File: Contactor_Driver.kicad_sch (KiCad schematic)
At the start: 26 parts, among them J1 Conn_01x04, Q3 BUK9M23-80E, Q4 FDC2512, Q5 NTR4003NT1G, Q6 NMOS, U2 SI8261ABC-IS

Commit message: Added part numbers and datasheet to isolator part
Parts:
- Q5: P/N (none) -> NTR4003NT1G
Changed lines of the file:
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@@
       (effects (font (size 1.27 1.27)) hide)
     )
-    (property "Datasheet" "~" (at 50.8 77.47 0)
+    (property "Datasheet" "https://www.mouser.com/datasheet/2/308/1/NTR4003N_D-2319203.pdf" (at 50.8 77.47 0)
       (effects (font (size 1.27 1.27)) hide)
     )
+    (property "P/N" "NTR4003NT1G" (at 50.8 77.47 0)
+      (effects (font (size 1.27 1.27)) hide)
+    )

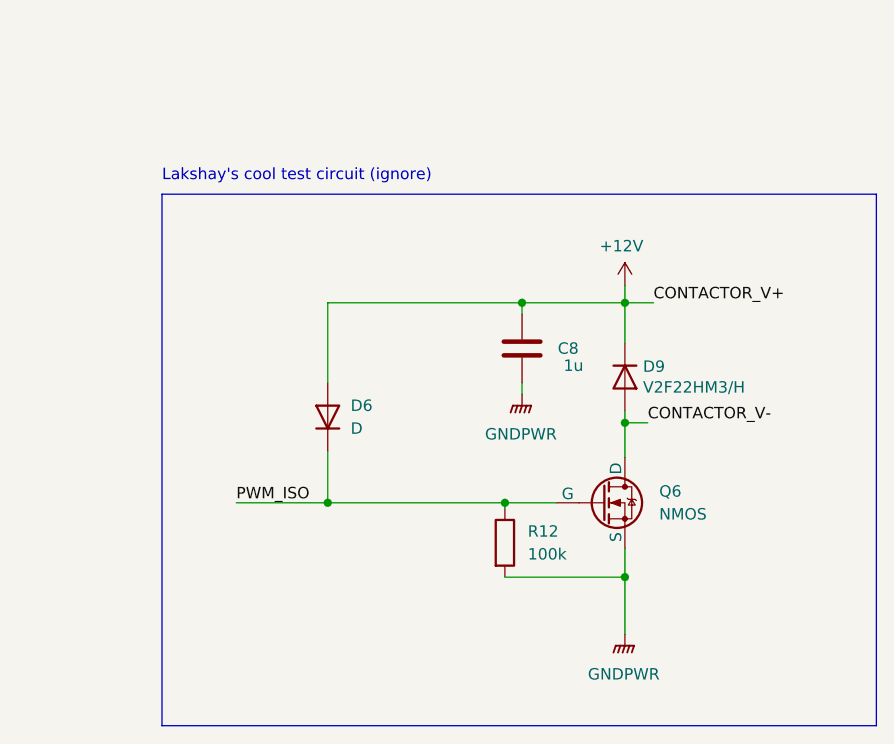
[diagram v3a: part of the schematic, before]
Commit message: removed redundant contactor circuit
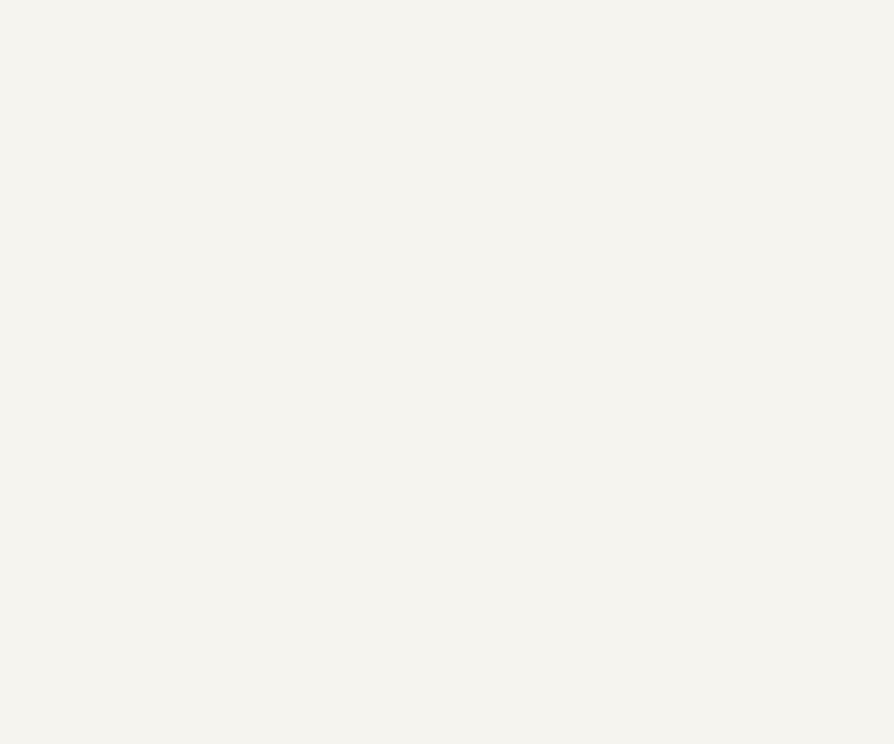
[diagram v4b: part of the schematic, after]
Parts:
- removed C8: 1u, Capacitor_SMD:C_0805_2012Metric, symbol Device:C
- removed D6: D, LED_SMD:LED_0805_2012Metric, symbol Device:D
- removed D9: V2F22HM3/H, UTSVT_Passive:V2F22HM, symbol Device:D
- removed Q6: NMOS, symbol Simulation_SPICE:NMOS
- removed R12: 100k, Resistor_SMD:R_0805_2012Metric, symbol Device:R
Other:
- note removed: "Lakshay's cool test circuit (ignore)"
